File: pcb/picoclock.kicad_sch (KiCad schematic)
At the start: 54 parts, among them J1 UART, J10 USB, J2 AUDIO, J3 xx, J4 xx, J5 Power In, J6 USB_C_Receptacle, J7 xx, J8 xx, J9 screen_adapter_connector, SW1 SW_Push, SW2 SW_Push, SW3 SW_Push, SW4 SW_Push, SW5 SW_Push, SW6 SW_Push, U1 PCF8563T, U2 Pico, U3 MCP9808_MSOP, U4 PCM5100, Y1 Crystal

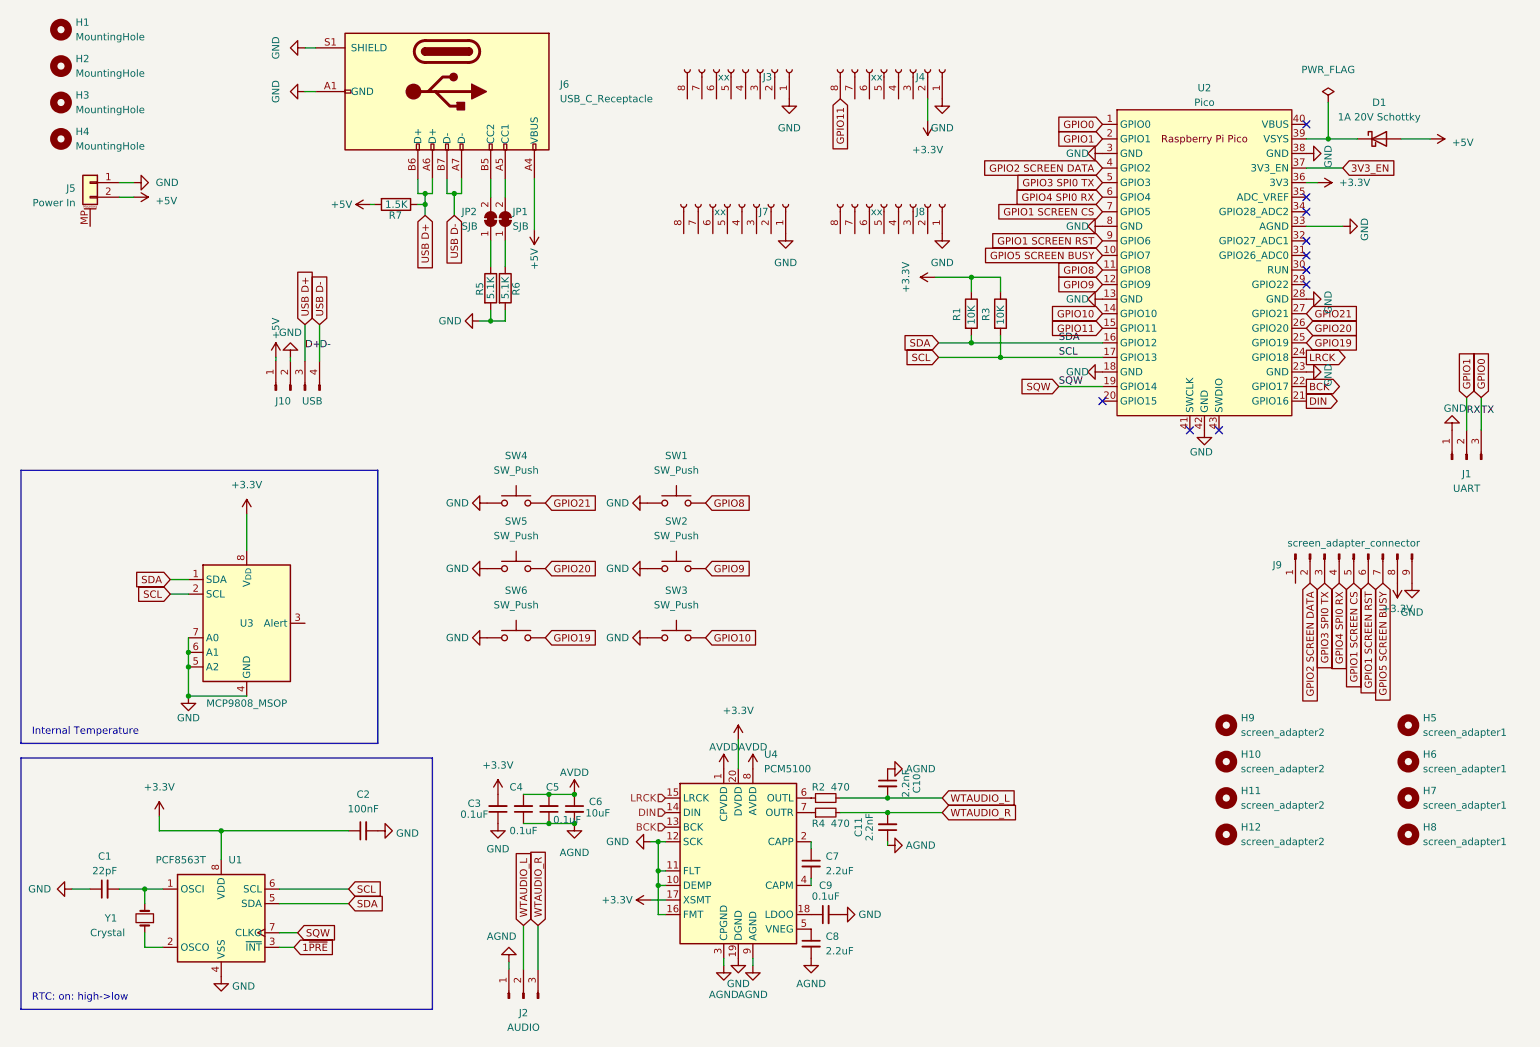
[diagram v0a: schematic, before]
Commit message: update case+pcb
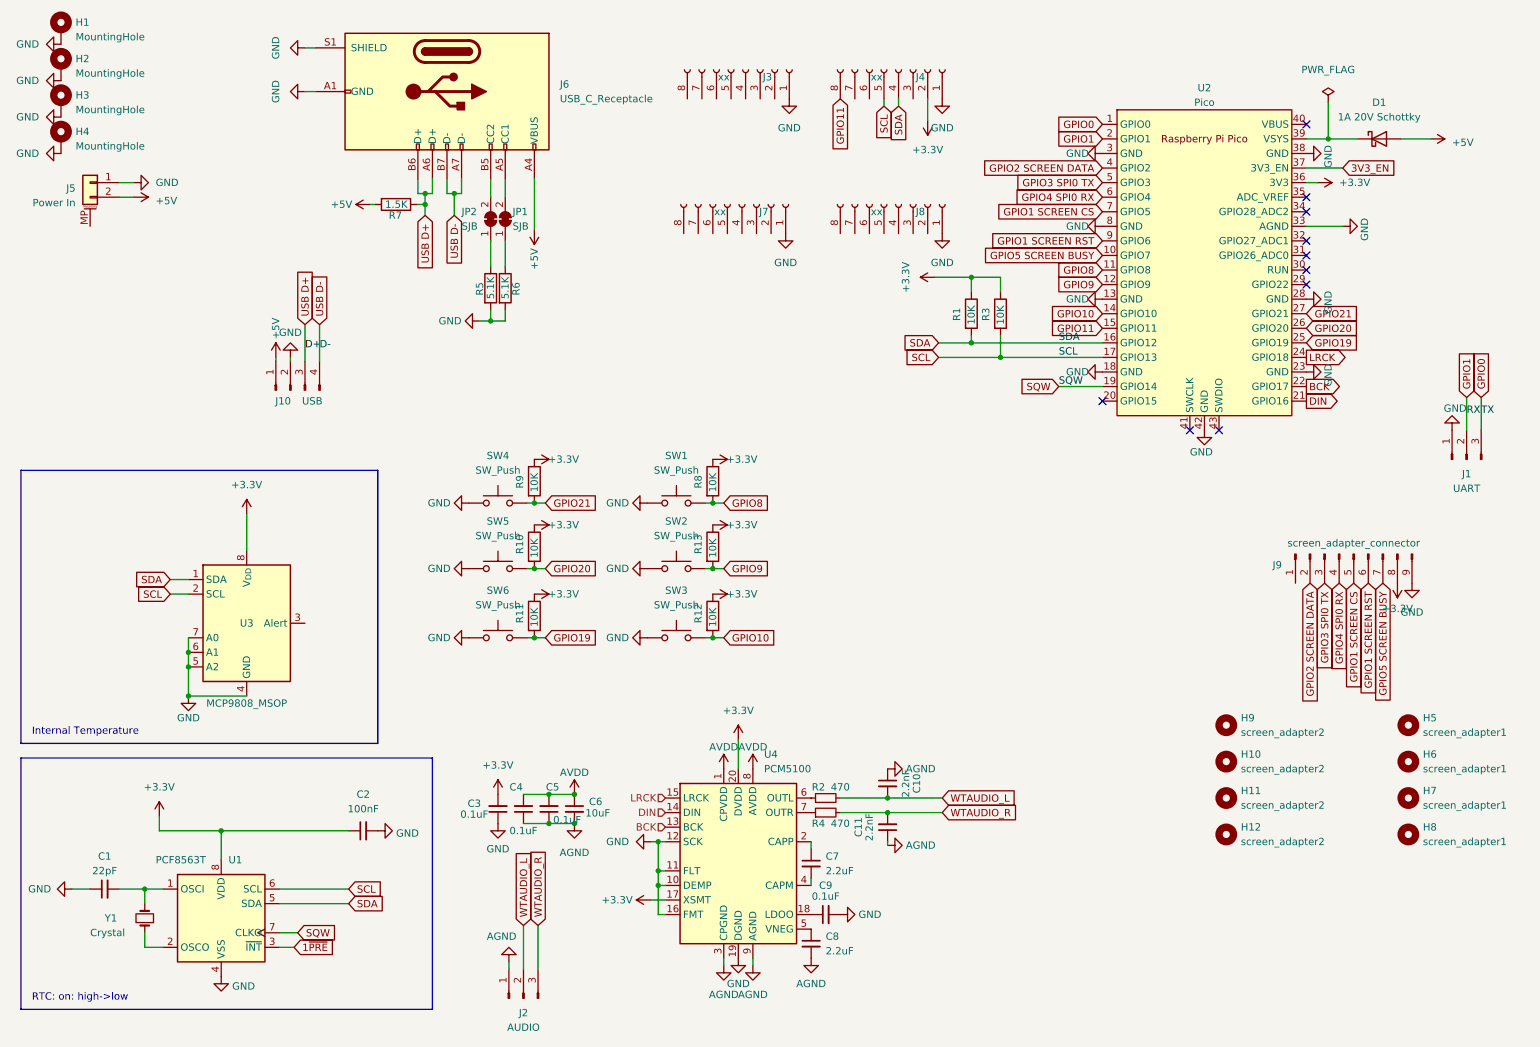
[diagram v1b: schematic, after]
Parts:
- added R10, R11, R12, R13, R8, R9: 10K, Resistor_SMD:R_0603_1608Metric, symbol Device:R
- H1, H2, H3, H4: footprint MountingHole:MountingHole_2.5mm -> MountingHole:MountingHole_3mm_Pad; symbol Mechanical:MountingHole -> Mechanical:MountingHole_Pad
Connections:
- net +3.3V: now also R10.1, R11.1, R12.1, R13.1, R8.1, R9.1
- net GND: now also H1.1, H2.1, H3.1, H4.1
- net GPIO10: now also R12.2
- net GPIO19: now also R11.2
- net GPIO20: now also R10.2
- net GPIO21: now also R9.2
- net GPIO8: now also R8.2
- net GPIO9: now also R13.2
- net SCL: now also J4.5 (Pin_5)
- net SDA: now also J4.4 (Pin_4)
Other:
- moved on the sheet: SW4, SW5, SW6

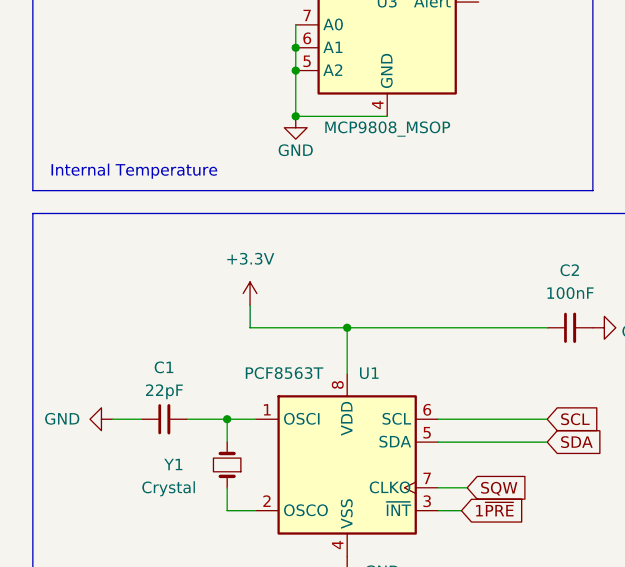
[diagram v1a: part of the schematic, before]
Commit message: [pcb] update
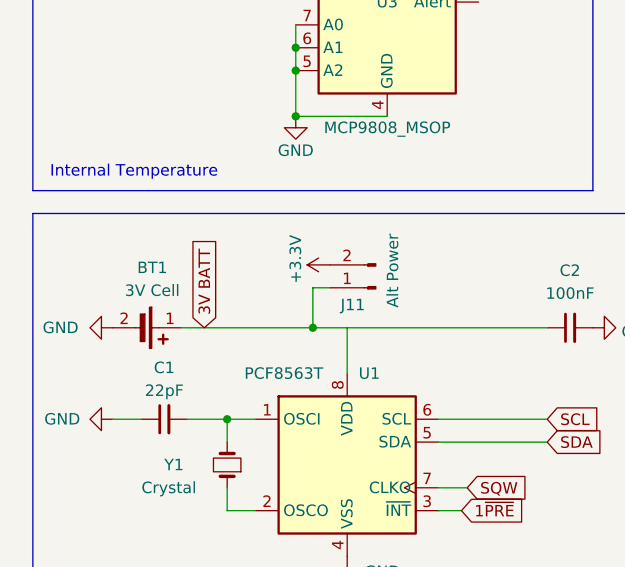
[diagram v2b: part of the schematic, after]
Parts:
- added BT1: 3V Cell, cell:MPD_BC501SM-TR, symbol Device:Battery_Cell
- added J11: Alt Power, Connector_PinHeader_2.54mm:PinHeader_1x02_P2.54mm_Vertical, symbol Connector:Conn_01x02_Pin
- C1, C2, C3, C4, C5, C9: footprint Capacitor_SMD:C_0402_1005Metric -> Capacitor_SMD:C_0603_1608Metric
- R2, R4: footprint Resistor_SMD:R_0402_1005Metric -> Resistor_SMD:R_0603_1608Metric
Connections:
- net +3.3V: now also J11.2 (Pin_2); no longer C2.1, U1.8 (VDD)
- net GND: now also BT1.2 (-)
- new net 3V BATT: BT1.1 (+), C2.1, J11.1 (Pin_1), U1.8 (VDD)
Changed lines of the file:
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@@
   (junction (at 243.84 40.64) (diameter 0) (color 0 0 0 0)
   )
+  (junction (at 46.99 161.29) (diameter 0) (color 0 0 0 0)
+  )
   (junction (at 45.085 132.715) (diameter 0) (color 0 0 0 0)
   )
@@
   (junction (at 107.95 160.02) (diameter 0) (color 0 0 0 0)
   )
-  (junction (at 50.8 161.29) (diameter 0) (color 0 0 0 0)
-  )
   (junction (at 37.465 171.45) (diameter 0) (color 0 0 0 0)
   )
@@
     (stroke (width 0) (type default))
   )
+  (wire (pts (xy 46.99 161.29) (xy 50.8 161.29))
+    (stroke (width 0) (type default))
+  )
   (wire (pts (xy 90.17 47.625) (xy 90.17 50.165))
     (stroke (width 0) (type default))
   )
-  (wire (pts (xy 40.005 161.29) (xy 50.8 161.29))
+  (wire (pts (xy 32.385 161.29) (xy 46.99 161.29))
     (stroke (width 0) (type default))
   )
@@
     (stroke (width 0) (type default))
   )
+  (wire (pts (xy 46.99 156.845) (xy 46.99 161.29))
+    (stroke (width 0) (type default))
+  )
   (wire (pts (xy 86.36 50.165) (xy 87.63 50.165))
     (stroke (width 0) (type default))
@@
     (stroke (width 0) (type default))
   )
+  (wire (pts (xy 46.99 156.845) (xy 48.895 156.845))
+    (stroke (width 0) (type default))
+  )
   (wire (pts (xy 100.33 70.485) (xy 100.33 72.39))
     (stroke (width 0) (type default))
@@
     (stroke (width 0) (type default))
   )
-  (wire (pts (xy 40.005 161.29) (xy 40.005 158.75))
-    (stroke (width 0) (type default))
-  )
   (wire (pts (xy 95.885 72.39) (xy 97.79 72.39))
     (stroke (width 0) (type default))
@@
     )
   )
+  (global_label "3V BATT" (shape input) (at 34.925 161.29 90) (fields_autoplaced)
+    (effects (font (size 1.27 1.27)) (justify left))
+    (property "Intersheetrefs" "${INTERSHEET_REFS}" (at 34.925 150.7453 90)
+      (effects (font (size 1.27 1.27)) (justify left) hide)
+    )
+  )
   (global_label "GPIO2 SCREEN DATA" (shape input) (at 240.665 118.11 270) (fields_autoplaced)
     (effects (font (size 1.27 1.27)) (justify right))
@@
     (effects (font (size 1.27 1.27)) (justify right))
   )
+  (symbol (lib_id "Device:Battery_Cell") (at 27.305 161.29 270) (unit 1)
+    (in_bom yes) (on_board yes) (dnp no) (fields_autoplaced)
+    (property "Reference" "BT1" (at 29.1465 154.6225 90)
+      (effects (font (size 1.27 1.27)))
+    )
+    (property "Value" "3V Cell" (at 29.1465 157.1625 90)
+      (effects (font (size 1.27 1.27)))
+    )
+    (property "Footprint" "cell:MPD_BC501SM-TR" (at 28.829 161.29 90)
+      (effects (font (size 1.27 1.27)) hide)
+    )
+    (property "Datasheet" "~" (at 28.829 161.29 90)
+      (effects (font (size 1.27 1.27)) hide)
+    )
+    (pin "2")
+    (pin "1")
+    (instances
+      (project "picoclock"
+        (path "/3b9dec0e-e0b7-4565-afc9-c4692f41aea9"
+          (reference "BT1") (unit 1)
+        )
+      )
+    )
+  )
   (symbol (lib_id "Device:R") (at 136.525 100.33 0) (unit 1)
     (in_bom yes) (on_board yes) (dnp no)
@@
     )
   )
+  (symbol (lib_id "power:+3.3V") (at 48.895 154.305 90) (unit 1)
+    (in_bom yes) (on_board yes) (dnp no)
+    (property "Reference" "#PWR03" (at 52.705 154.305 0)
+      (effects (font (size 1.27 1.27)) hide)
+    )
+    (property "Value" "+3.3V" (at 45.085 153.67 0)
+      (effects (font (size 1.27 1.27)))
+    )
+    (property "Footprint" "" (at 48.895 154.305 0)
+      (effects (font (size 1.27 1.27)) hide)
+    )
+    (property "Datasheet" "" (at 48.895 154.305 0)
+      (effects (font (size 1.27 1.27)) hide)
+    )
+    (pin "1")
+    (instances
+      (project "picoclock"
+        (path "/3b9dec0e-e0b7-4565-afc9-c4692f41aea9"
+          (reference "#PWR03") (unit 1)
+        )
+      )
+    )
+  )
   (symbol (lib_id "power:+3.3V") (at 136.525 120.015 270) (unit 1)
     (in_bom yes) (on_board yes) (dnp no)
@@
       (effects (font (size 1.27 1.27)))
     )
-    (property "Footprint" "Capacitor_SMD:C_0402_1005Metric" (at 99.06 157.48 0)
+    (property "Footprint" "Capacitor_SMD:C_0603_1608Metric" (at 99.06 157.48 0)
       (effects (font (size 1.27 1.27)) hide)
     )
@@
       (effects (font (size 1.27 1.27)))
     )
-    (property "Footprint" "Capacitor_SMD:C_0402_1005Metric" (at 156.21 175.895 0)
+    (property "Footprint" "Capacitor_SMD:C_0603_1608Metric" (at 156.21 175.895 0)
       (effects (font (size 1.27 1.27)) hide)
     )
@@
       (effects (font (size 1.27 1.27)))
     )
-    (property "Footprint" "Resistor_SMD:R_0402_1005Metric" (at 156.21 158.115 0)
+    (property "Footprint" "Resistor_SMD:R_0603_1608Metric" (at 156.21 158.115 0)
       (effects (font (size 1.27 1.27)) hide)
     )
@@
     )
   )
+  (symbol (lib_id "power:GND") (at 24.765 161.29 270) (unit 1)
+    (in_bom yes) (on_board yes) (dnp no) (fields_autoplaced)
+    (property "Reference" "#PWR069" (at 18.415 161.29 0)
+      (effects (font (size 1.27 1.27)) hide)
+    )
+    (property "Value" "GND" (at 20.955 161.29 90)
+      (effects (font (size 1.27 1.27)) (justify right))
+    )
+    (property "Footprint" "" (at 24.765 161.29 0)
+      (effects (font (size 1.27 1.27)) hide)
+    )
+    (property "Datasheet" "" (at 24.765 161.29 0)
+      (effects (font (size 1.27 1.27)) hide)
+    )
+    (pin "1")
+    (instances
+      (project "picoclock"
+        (path "/3b9dec0e-e0b7-4565-afc9-c4692f41aea9"
+          (reference "#PWR069") (unit 1)
+        )
+      )
+    )
+  )
   (symbol (lib_id "Device:C_Small") (at 153.67 167.005 0) (unit 1)
     (in_bom yes) (on_board yes) (dnp no) (fields_autoplaced)
@@
       (effects (font (size 1.27 1.27)))
     )
-    (property "Footprint" "Capacitor_SMD:C_0402_1005Metric" (at 103.505 157.48 0)
+    (property "Footprint" "Capacitor_SMD:C_0603_1608Metric" (at 103.505 157.48 0)
       (effects (font (size 1.27 1.27)) hide)
     )
@@
     )
   )
-  (symbol (lib_id "power:+3.3V") (at 40.005 158.75 0) (unit 1)
-    (in_bom yes) (on_board yes) (dnp no) (fields_autoplaced)
-    (property "Reference" "#PWR03" (at 40.005 162.56 0)
-      (effects (font (size 1.27 1.27)) hide)
-    )
-    (property "Value" "+3.3V" (at 40.005 153.67 0)
-      (effects (font (size 1.27 1.27)))
-    )
-    (property "Footprint" "" (at 40.005 158.75 0)
-      (effects (font (size 1.27 1.27)) hide)
-    )
-    (property "Datasheet" "" (at 40.005 158.75 0)
-      (effects (font (size 1.27 1.27)) hide)
-    )
-    (pin "1")
-    (instances
-      (project "picoclock"
-        (path "/3b9dec0e-e0b7-4565-afc9-c4692f41aea9"
-          (reference "#PWR03") (unit 1)
-        )
-      )
-    )
-  )
   (symbol (lib_id "power:+5V") (at 105.41 56.515 180) (unit 1)
     (in_bom yes) (on_board yes) (dnp no)
@@
       (effects (font (size 1.27 1.27)))
     )
-    (property "Footprint" "Capacitor_SMD:C_0402_1005Metric" (at 30.48 171.45 0)
+    (property "Footprint" "Capacitor_SMD:C_0603_1608Metric" (at 30.48 171.45 0)
       (effects (font (size 1.27 1.27)) hide)
     )
@@
       (effects (font (size 1.27 1.27)))
     )
-    (property "Footprint" "Capacitor_SMD:C_0402_1005Metric" (at 75.565 161.29 0)
+    (property "Footprint" "Capacitor_SMD:C_0603_1608Metric" (at 75.565 161.29 0)
       (effects (font (size 1.27 1.27)) hide)
     )
@@
     )
   )
+  (symbol (lib_id "Connector:Conn_01x02_Pin") (at 53.975 156.845 180) (unit 1)
+    (in_bom yes) (on_board yes) (dnp no)
+    (property "Reference" "J11" (at 51.435 158.75 0)
+      (effects (font (size 1.27 1.27)))
+    )
+    (property "Value" "Alt Power" (at 55.88 154.94 90)
+      (effects (font (size 1.27 1.27)))
+    )
+    (property "Footprint" "Connector_PinHeader_2.54mm:PinHeader_1x02_P2.54mm_Vertical" (at 53.975 156.845 0)
+      (effects (font (size 1.27 1.27)) hide)
+    )
+    (property "Datasheet" "~" (at 53.975 156.845 0)
+      (effects (font (size 1.27 1.27)) hide)
+    )
+    (pin "1")
+    (pin "2")
+    (instances
+      (project "picoclock"
+        (path "/3b9dec0e-e0b7-4565-afc9-c4692f41aea9"
+          (reference "J11") (unit 1)
+        )
+      )
+    )
+  )
   (symbol (lib_id "Connector:Conn_01x08_Socket") (at 168.91 28.575 270) (mirror x) (unit 1)
     (in_bom yes) (on_board yes) (dnp no)
@@
       (effects (font (size 1.27 1.27)))
     )
-    (property "Footprint" "Resistor_SMD:R_0402_1005Metric" (at 156.21 155.575 0)
+    (property "Footprint" "Resistor_SMD:R_0603_1608Metric" (at 156.21 155.575 0)
       (effects (font (size 1.27 1.27)) hide)
     )
@@
       (effects (font (size 1.27 1.27)))
     )
-    (property "Footprint" "Capacitor_SMD:C_0402_1005Metric" (at 107.95 157.48 0)
+    (property "Footprint" "Capacitor_SMD:C_0603_1608Metric" (at 107.95 157.48 0)
       (effects (font (size 1.27 1.27)) hide)
     )
